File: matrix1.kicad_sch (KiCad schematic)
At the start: 5 parts, among them U5 MAX7221CWG+T

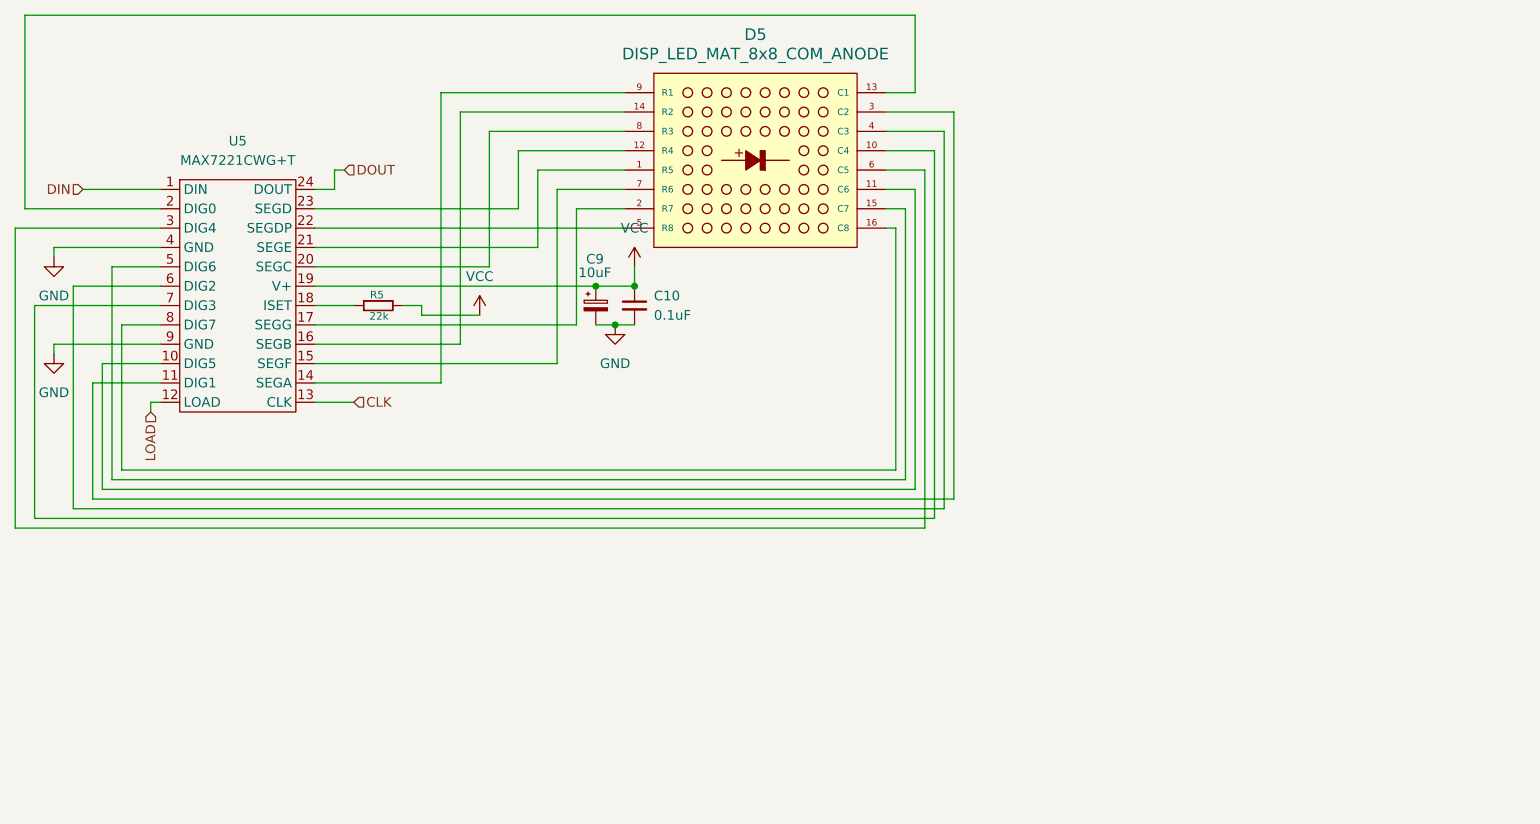
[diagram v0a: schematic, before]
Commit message: Added PDF schema
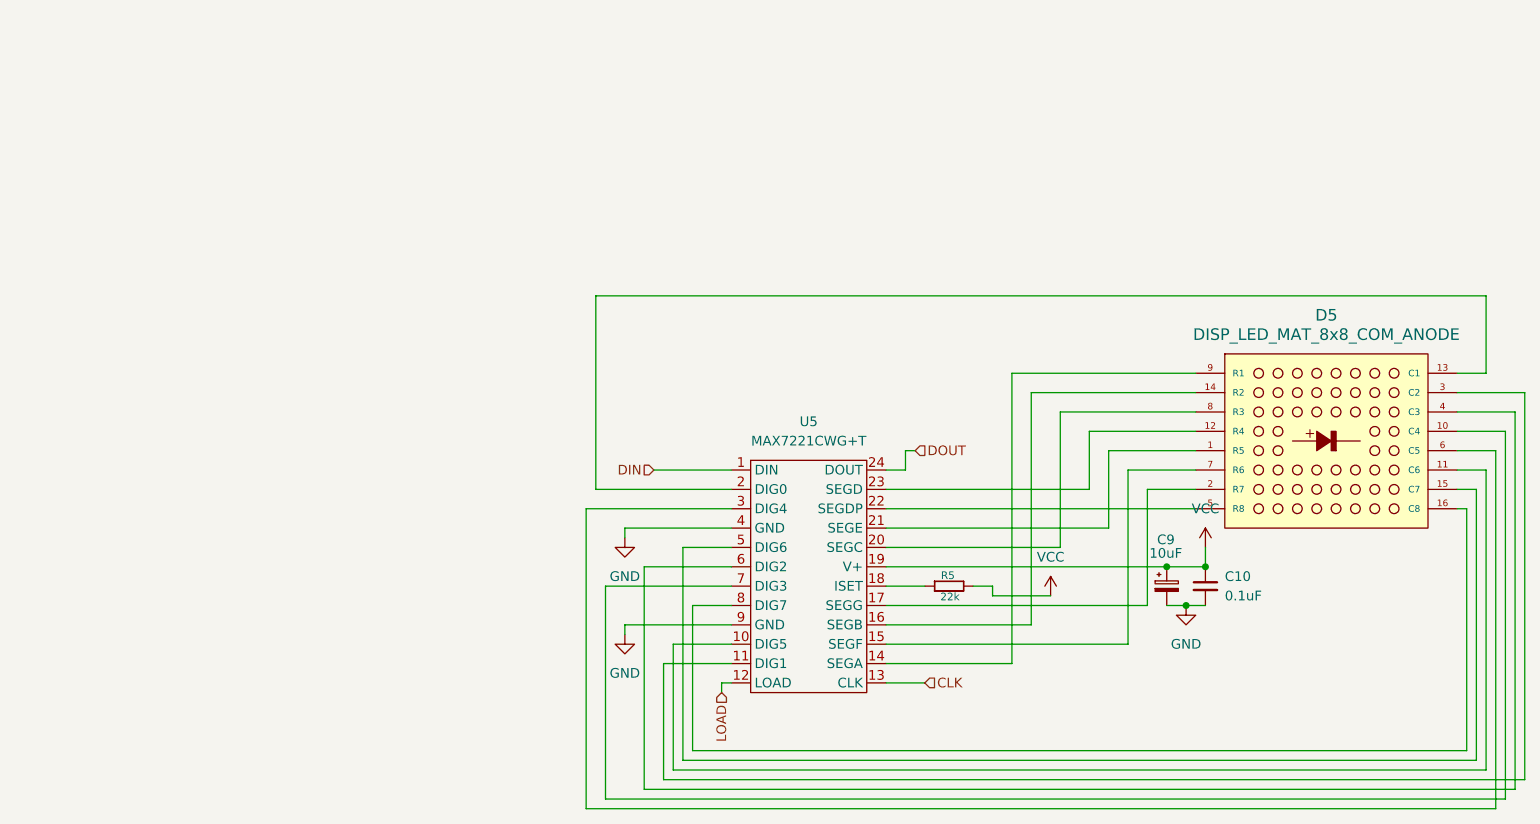
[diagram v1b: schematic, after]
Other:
- title: (none) -> esp32c3 Led Matrix 6x8x8 - Matrix Schema
- moved on the sheet: C10, C9, D5, R5, U5
